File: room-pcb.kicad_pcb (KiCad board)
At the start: 4 copper layers, 50 x 50 mm, 28 parts, among them J1 Conn_01x08, J2 Conn_01x02, J3 Conn_01x04, U1 COZIR, U2 BH1750FVI-TR, U3 AHT20, U4 LD2450, U5 ESP32-C6_SUPERMINI_TH

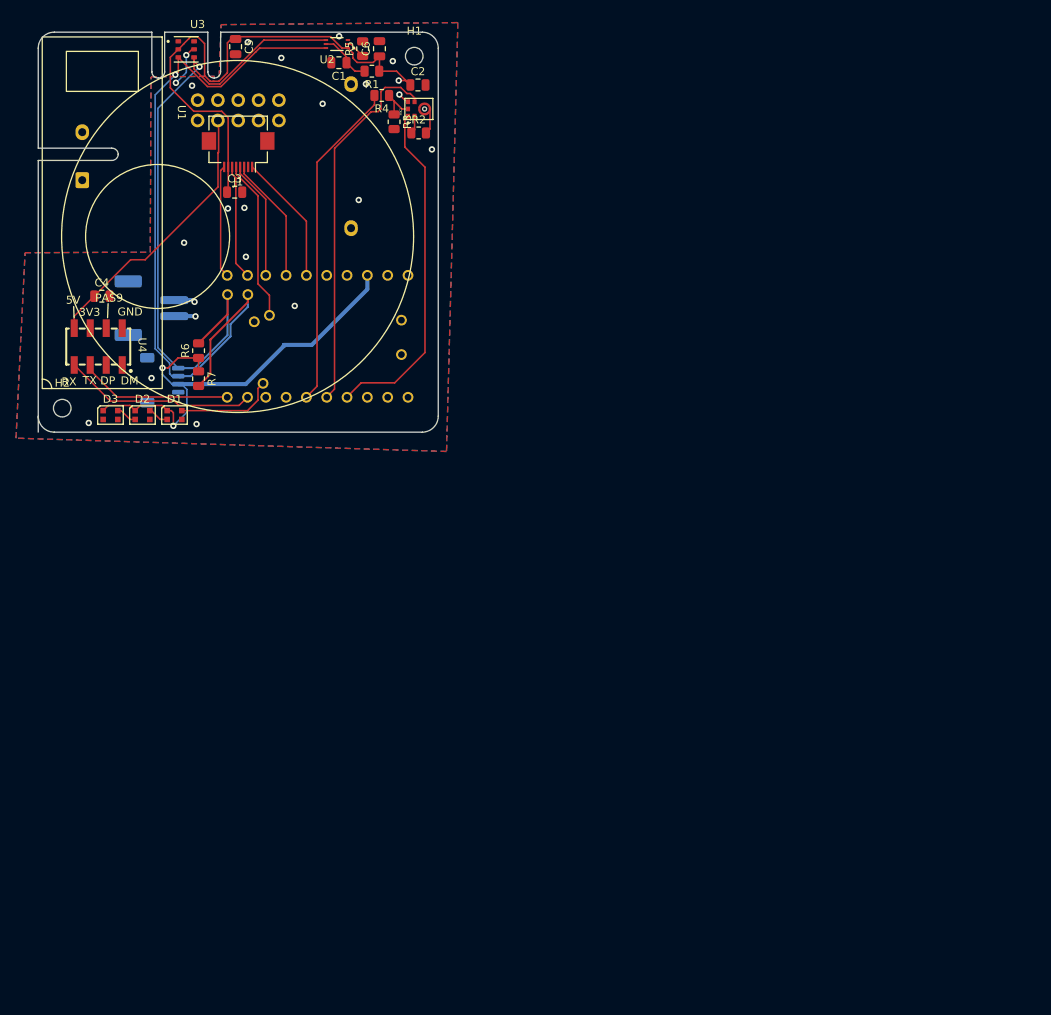
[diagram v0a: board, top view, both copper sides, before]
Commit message: new layout
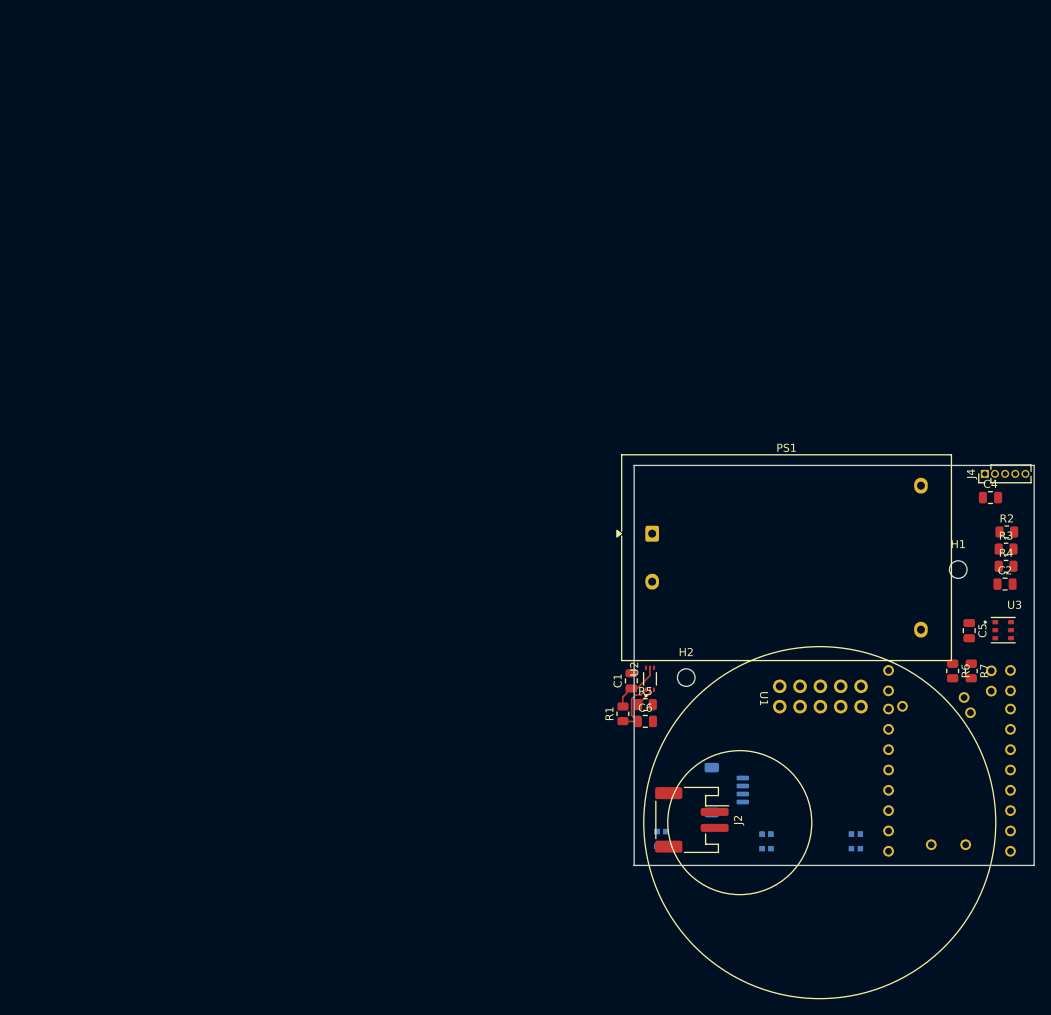
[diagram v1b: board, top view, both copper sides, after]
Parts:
- removed C3: 0.1U, Capacitor_SMD:C_0805_2012Metric
- removed J1: Conn_01x08, Connector_FFC-FPC:Hirose_FH12-8S-0.5SH_1x08-1MP_P0.50mm_Horizontal
- removed MK1: ICS-43434, ICS-43434:MIC_ICS-43434
- removed U4: LD2450, ld2450:ld2450
- added J4: Conn_01x05, Connector_PinHeader_1.27mm:PinHeader_1x05_P1.27mm_Vertical, F.Cu at (143.3, 80.2)
- D1, D2, D3: moved to B.Cu
- J2, PS1: moved to F.Cu
- moved U3 125.3 mm to (145.6, 99.8)
- moved C5 117.2 mm to (141.4, 99.8)
- moved C4 113.9 mm to (144.0, 83.2)
- moved R7 103.3 mm to (141.6, 104.8)
- moved U1 103.3 mm to (117.7, 109.3)
- moved R6 102.4 mm to (139.3, 104.8), turned to -90 degrees
- moved D1 100.5 mm to (127.2, 126.2), turned to 90 degrees
- moved R4 97.7 mm to (146.0, 91.8), turned to 0 degrees
- moved C2 96.3 mm to (145.8, 94.0)
- moved U5 94.8 mm to (138.9, 117.7), turned to 0 degrees
- moved D2 94.5 mm to (116.0, 126.2), turned to 90 degrees
- moved H1 93.5 mm to (140.0, 92.2)
- moved R3 93.3 mm to (146.0, 89.6), turned to 0 degrees
- moved J2 93.0 mm to (106.7, 123.5), turned to -90 degrees
- moved C6 90.4 mm to (100.9, 111.2), turned to 0 degrees
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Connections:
- U5 pad 14: DC -> unconnected-(U5-GPIO14-Pad14)
- U5 pad 15: RST -> unconnected-(U5-GPIO15-Pad15)
- U5 pad 18: BL -> unconnected-(U5-GPIO18-Pad18)
- U5 pad 21: MOSI -> unconnected-(U5-GPIO21-Pad21)
- U5 pad 9: SCK -> unconnected-(U5-GPIO9-Pad9)
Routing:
- net +3.3V: track 212.6 -> 7.25 mm, vias 4 -> 0
- net SCL: track 93.6 -> 0.00 mm, vias 1 -> 0
- net SDA: track 83.9 -> 0.00 mm, vias 1 -> 0
- net VCC: track 80.3 -> 0.00 mm
- net CLK: track 46.9 -> 0.00 mm
- net CAL: track 42.9 -> 0.00 mm
- net WS: track 42.8 -> 0.00 mm
- net DATA: track 41.2 -> 0.00 mm
- net BAT-: track 34.7 -> 0.00 mm, vias 1 -> 0
- net BAT+: track 31.1 -> 0.00 mm, vias 1 -> 0
- net RX1: track 24.2 -> 0.00 mm
- net TX: track 23.9 -> 0.00 mm
- net RX: track 23.9 -> 0.00 mm
- net MOSI: track 20.3 -> 0.00 mm
- net TX1: track 19.2 -> 0.00 mm
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- removed copper zone on B.Cu, net GND
- removed copper zone on F.Cu, net GND
- removed copper zone on In1.Cu, net GND
- removed copper zone on In2.Cu, net GND
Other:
- outline, holes or cut-outs redrawn
